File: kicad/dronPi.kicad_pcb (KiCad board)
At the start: 2 copper layers, 140 parts, among them IC1 MIC5332, IC10 24AA32, IC11 MAX3370, IC12 SN74LVC1G07, IC2 MPU-9250, IC3 MS5611-01BA, IC4 PCA9306, IC5 ADC_ADS1115, IC6 PCA9685, IC7 BQ24315, IC8 MCP2515, IC9 MCP2551, J1 RPi_GPIO, M1 OSHW-LOGOS, P1 CONN_3X16, P2 PowerOff, Q1 MMBT3906LT1, Q2 DMG2305, U1 DMMT5401

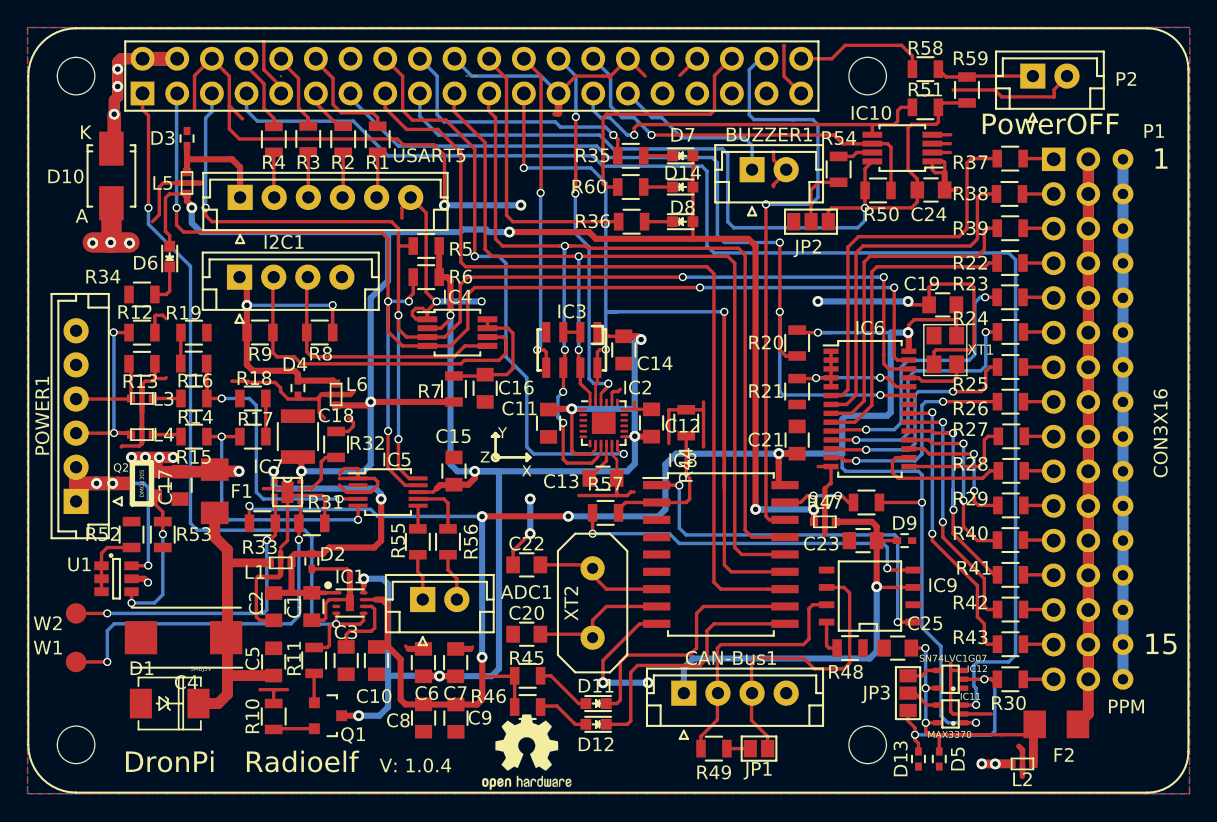
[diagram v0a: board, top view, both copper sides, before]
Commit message: V1.0.5
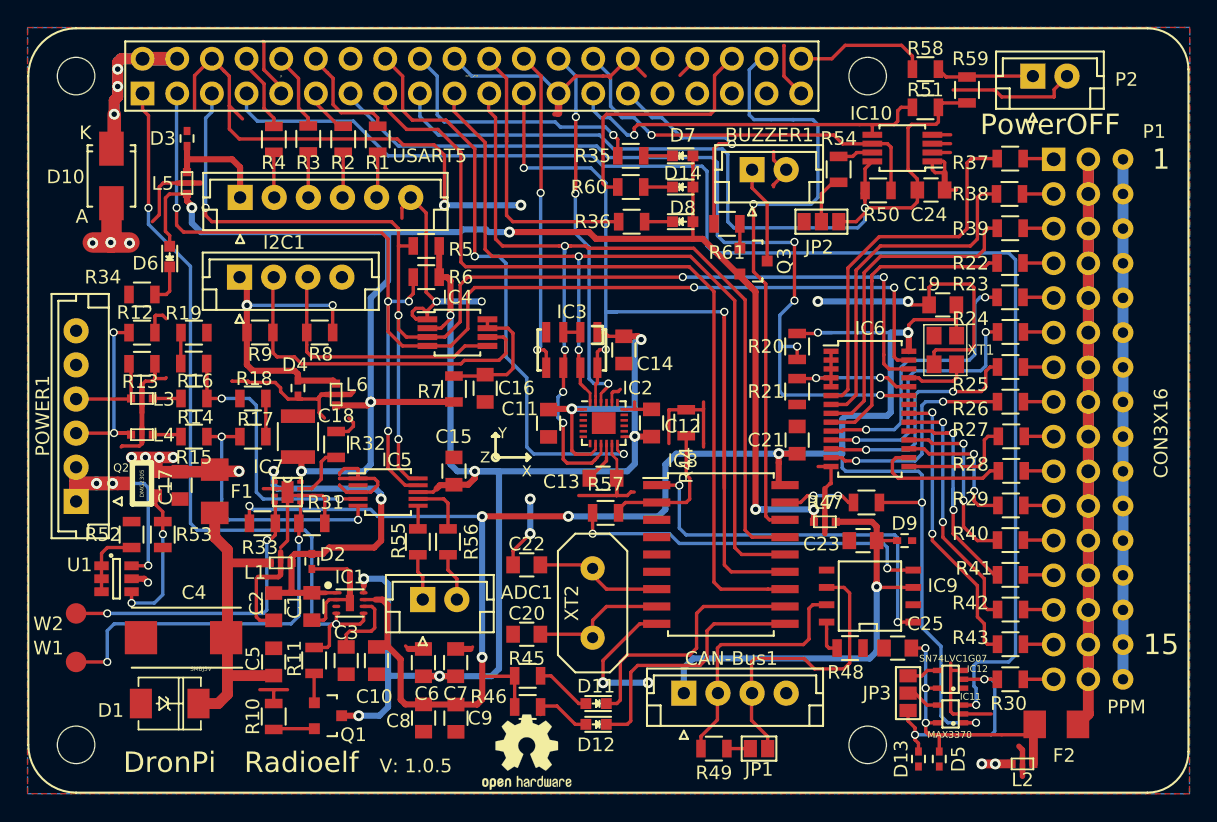
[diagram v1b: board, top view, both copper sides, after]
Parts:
- added Q3: MMBT3906, TO_SOT_Packages_SMD:SOT-23, F.Cu at (160.1, 91.3)
- added R61: 1K, Resistors_SMD:R_0805, F.Cu at (158.2, 88.5)
- moved JP2 0.76 mm to (165.1, 88.4)
- moved R20 0.25 mm to (163.3, 97.5)
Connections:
- BUZZER1 pad 1: BUZZER -> Net-(BUZZER1-Pad1)
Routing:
- net Net-(BUZZER1-Pad1): track 0.00 -> 7.15 mm
- net BUZZER: track 12.5 -> 16.2 mm, vias 0 -> 1
- net SPI_MISO: track 73.8 -> 71.9 mm
- net Net-(Q3-Pad1): track 0.00 -> 1.78 mm
- net SPI_MOSI: track 67.1 -> 65.5 mm
- net SPI_CS_CAN: track 44.1 -> 45.4 mm
- net 3v3: track 65.0 -> 64.0 mm
- net Net-(IC6-Pad6): track 28.3 -> 27.4 mm
- net Net-(JP2-Pad2): track 4.46 -> 3.64 mm
- net INT_CAN: track 63.5 -> 62.8 mm
- net Net-(IC6-Pad7): track 26.4 -> 25.7 mm
- net VCC_AUX: track 114.2 -> 113.6 mm
- net PWM_EN: track 64.0 -> 63.6 mm, vias 3 -> 4
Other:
- board text added: "V: 1.0.5"
- board text removed: "V: 1.0.4"
